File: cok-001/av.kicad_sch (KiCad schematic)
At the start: 81 parts, among them J2401 AV OUT, Q2401 DTC144E, Q2402 SI2303BDS, Q2403 IMH20T108, Q2404 DTA144E, U2402 MC78M09, U2403 MC78M05, U2405 CX4351

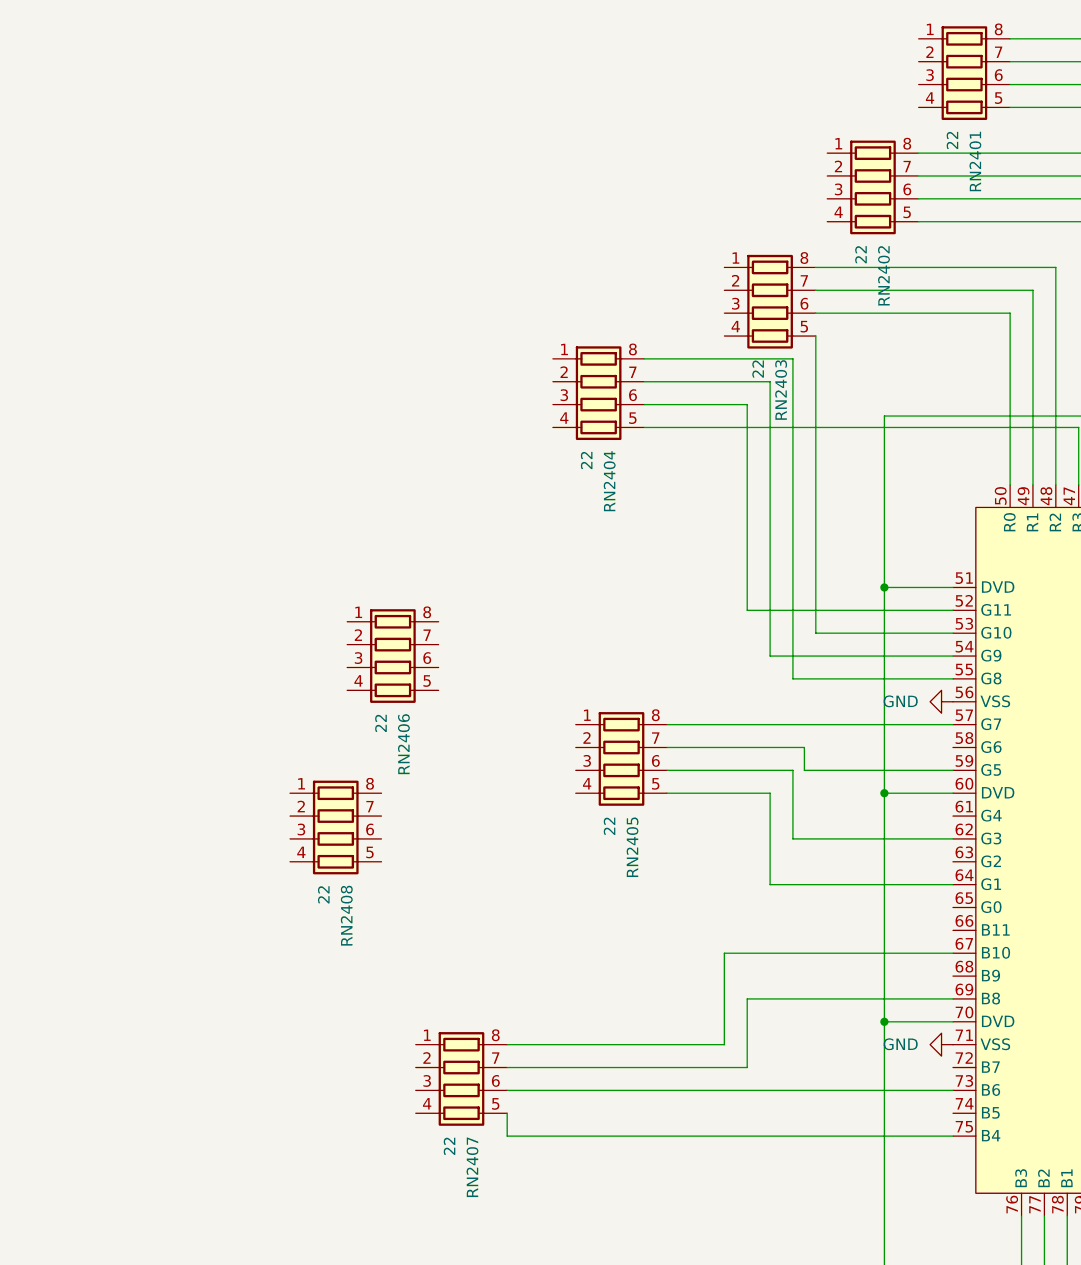
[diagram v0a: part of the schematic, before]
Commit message: rsx vo
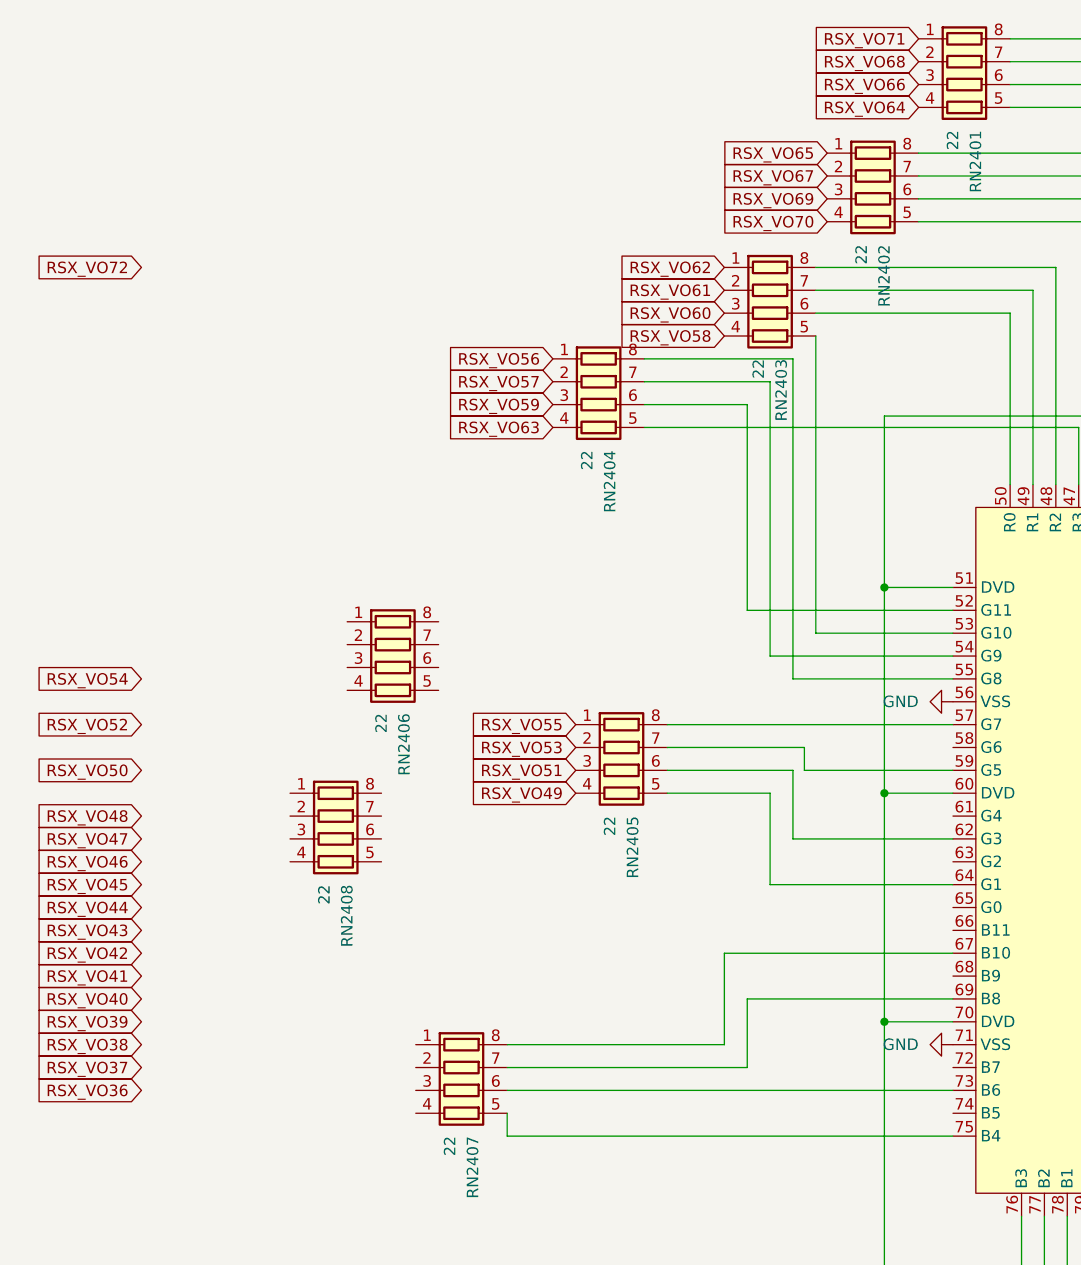
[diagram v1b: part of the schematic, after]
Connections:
- net RSX_VO65: now reaches RN2402.1 (R1.1)
- net RSX_VO67: now reaches RN2402.2 (R2.1)
- net RSX_VO69: now reaches RN2402.3 (R3.1)
- net RSX_VO70: now reaches RN2402.4 (R4.1)
- net RSX_VO56: now reaches RN2404.1 (R1.1)
- net RSX_VO57: now reaches RN2404.2 (R2.1)
- net RSX_VO59: now reaches RN2404.3 (R3.1)
- net RSX_VO63: now reaches RN2404.4 (R4.1)
- net RSX_VO71: now reaches RN2401.1 (R1.1)
- net RSX_VO68: now reaches RN2401.2 (R2.1)
- net RSX_VO66: now reaches RN2401.3 (R3.1)
- net RSX_VO64: now reaches RN2401.4 (R4.1)
- net RSX_VO55: now reaches RN2405.1 (R1.1)
- net RSX_VO53: now reaches RN2405.2 (R2.1)
- net RSX_VO51: now reaches RN2405.3 (R3.1)
- net RSX_VO49: now reaches RN2405.4 (R4.1)
- net RSX_VO62: now reaches RN2403.1 (R1.1)
- net RSX_VO61: now reaches RN2403.2 (R2.1)
- net RSX_VO60: now reaches RN2403.3 (R3.1)
- net RSX_VO58: now reaches RN2403.4 (R4.1)
